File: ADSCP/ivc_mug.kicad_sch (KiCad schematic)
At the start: 12 parts, among them U1 TL074 or OPA1644, U3 TL074 or OPA1644

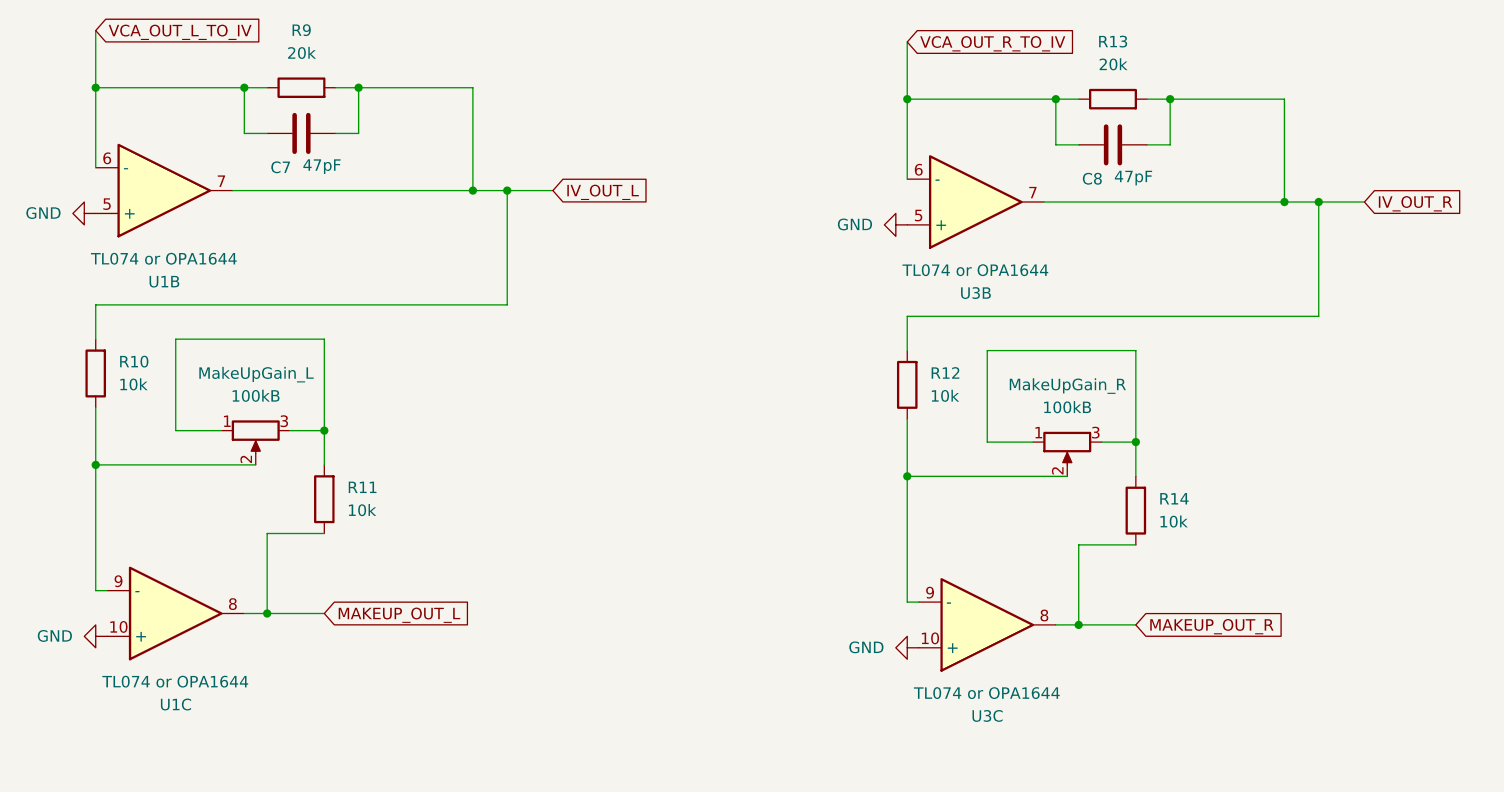
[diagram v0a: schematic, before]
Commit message: add schematics
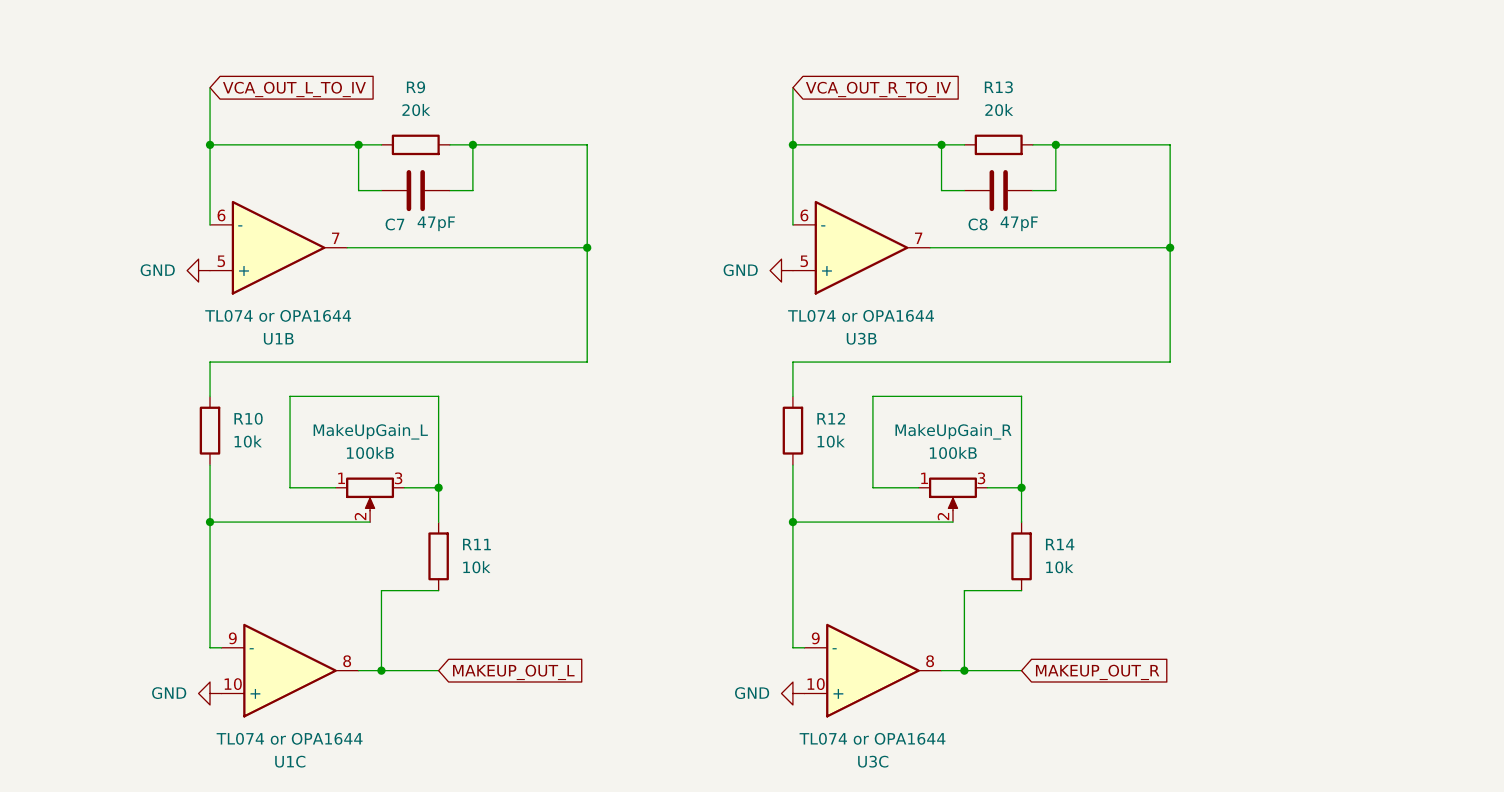
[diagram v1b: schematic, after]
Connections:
- net IV_OUT_L: no longer names the net of C7.1, R10.2, R9.2, U1.7
- net IV_OUT_R: no longer names the net of C8.1, R12.2, R13.2, U3.7
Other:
- moved on the sheet: C7, C8, MakeUpGain_L, MakeUpGain_R, R10, R11, R12, R13, R14, R9, U1B, U1C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
